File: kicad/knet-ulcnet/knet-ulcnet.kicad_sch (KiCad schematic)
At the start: 16 parts, among them U1 74LS157, U2 74LS00, U3 74LS139, U4 74LS86, U5 74LS74, U6 74LS74, U7 74LS123, U8 SN75176AP, U9 LM339

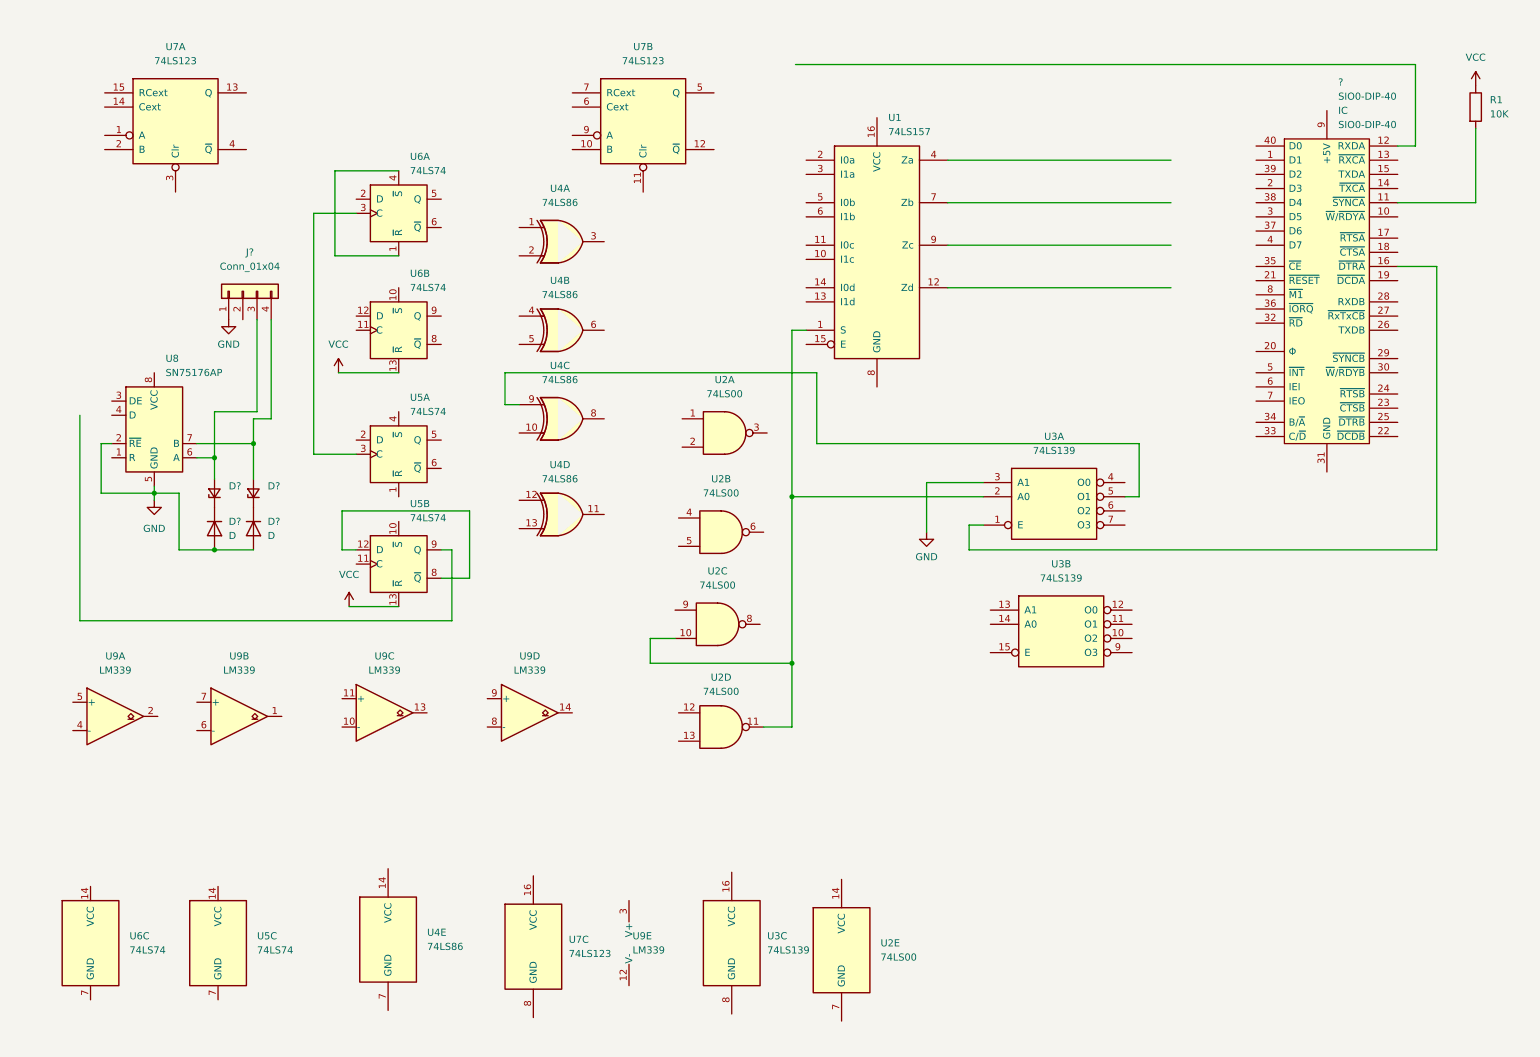
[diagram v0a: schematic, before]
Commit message: Update schematics etc for WEB-NT product
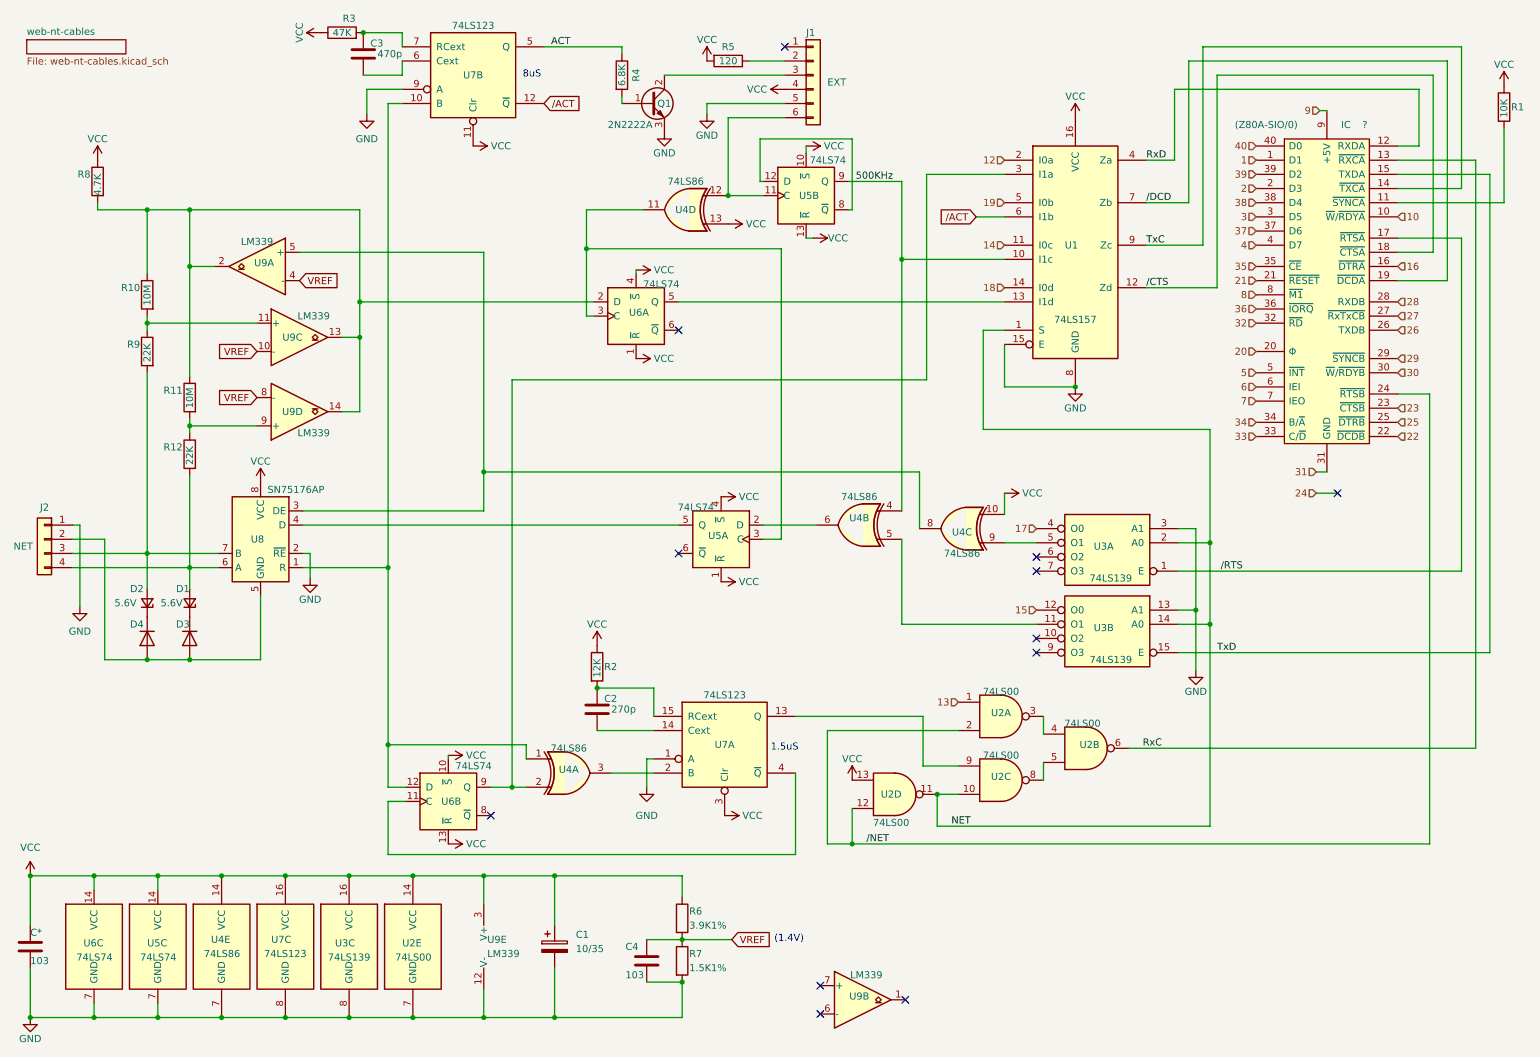
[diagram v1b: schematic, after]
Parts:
- added C*, C4: 103, symbol Device:C
- added C1: 10/35, symbol Device:C_Polarized
- added C2: 270p, symbol Device:C
- added C3: 470p, symbol Device:C
- added J1: EXT, symbol Connector_Generic:Conn_01x06
- added Q1: 2N2222A, symbol Device:Q_NPN_BCE
- added R10, R11: 10M, symbol Device:R
- added R12, R9: 22K, symbol Device:R
- added R2: 12K, symbol Device:R
- added R3: 47K, symbol Device:R
- added R4: 6.8K, symbol Device:R
- added R5: 120, symbol Device:R
- added R6: 3.9K1%, symbol Device:R
- added R7: 1.5K1%, symbol Device:R
- added R8: 4.7K, symbol Device:R
- ?: value SIO0-DIP-40 -> (none); Value_1 SIO0-DIP-40 -> (Z80A-SIO/0)
- D1, D2: renamed from D?; value (none) -> 5.6V
- D3, D4: renamed from D?; value D -> (none)
- J2: renamed from J?; value Conn_01x04 -> NET
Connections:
- net GND: now also U1.15 (E), U1.8 (GND), U2.7 (GND), U3.13 (A1), U3.8 (GND), U4.7 (GND), U5.7 (GND), U6.7 (GND), U7.1 (A), U7.8 (GND), U7.9 (A), U9.12 (V-), C*.2, C1.2, C4.2, J1.5 (Pin_5), Q1.3 (E), R7.2; no longer D3.2 (A), D4.2 (A), U8.5 (GND)
- net VCC: now also U1.16 (VCC), U2.13, U2.14 (VCC), U3.16 (VCC), U4.10, U4.13, U4.14 (VCC), U5.1 (~{R}), U5.10 (~{S}), U5.14 (VCC), U5.4 (~{S}), U6.1 (~{R}), U6.10 (~{S}), U6.14 (VCC), U6.4 (~{S}), U7.11 (Clr), U7.16 (VCC), U7.3 (Clr), U8.8 (VCC), U9.3 (V+), C*.1, C1.1, J1.4 (Pin_4), R2.1, R3.1, R5.2, R6.1, R8.1
- net NET: now reaches U1.1 (S), U2.10, U2.11, U3.2 (A0)
- net NET: now also U3.14 (A0)
- net 500KHz: now reaches U1.10 (I1c)
- net 500KHz: now also U4.4, U5.9 (Q)
- net 14: now reaches U1.11 (I0c)
- net /CTS: now reaches U1.12 (Zd)
- net /CTS: now also ?.18 (~{CTSA})
- net at U1.13 (I1d): now also U6.5 (Q)
- net 18: now reaches U1.14 (I0d)
- net 12: now reaches U1.2 (I0a)
- net at U1.3 (I1a): now also U4.2, U6.9 (Q)
- net RxD: now reaches U1.4 (Za)
- net RxD: now also ?.12 (RXDA)
- net 19: now reaches U1.5 (I0b)
- net /ACT: now reaches U1.6 (I1b)
- net /ACT: now also U7.12 (~{Q})
- net /DCD: now reaches U1.7 (Zb)
- net /DCD: now also ?.19 (~{DCDA})
- net TxC: now reaches U1.9 (Zc)
- net TxC: now also ?.14 (~{TXCA})
- net at D2.2 (A), U8.7 (B): now also J2.3 (Pin_3), R9.2; no longer J2.4 (Pin_4)
- net at U9.2: now also U6.2 (D), U9.13, U9.14, R10.1, R11.1, R8.2
- net VREF: now reaches U9.4 (-)
- net VREF: now also U9.10 (-), U9.8 (-), C4.1, R6.2, R7.1
- net at U9.5 (+): now also U4.8, U8.3 (DE)
- net at U3.11 (O1): now also U4.5
- net 15: now reaches U3.12 (O0)
- net TxD: now reaches U3.15 (E)
- net TxD: now also ?.15 (TXDA)
- net /NET: now reaches U2.12
- net /NET: now also ?.24 (~{RTSB}), U2.2
- net at U7.13 (Q): now also U2.9
- net at U7.14 (Cext): now also C2.2
- net at U7.15 (RCext): now also C2.1, R2.2
- net at U7.2 (B): now also U4.3
- net at U7.4 (~{Q}): now also U6.11 (C)
- net 13: now reaches U2.1
- net at U2.3: now also U2.4
- net at U4.11: now also U5.3 (C), U6.3 (C)
- net at U4.12: now also U5.11 (C), J1.6 (Pin_6)
- net at U6.12 (D): now also U4.1, U7.10 (B), U8.1 (R)
- net ACT: now reaches U7.5 (Q)
- net ACT: now also R4.1
- net at U7.6 (Cext): now also C3.2
- net at U7.7 (RCext): now also C3.1, R3.2
- net 1: now reaches ?.1 (D1)
- net 10: now reaches ?.10 (~{W}/~{RDYA})
- net RxC: now reaches ?.13 (~{RXCA})
- net RxC: now also U2.6
- net 16: now reaches ?.16 (~{DTRA})
- net 16: no longer U3.1 (E)
- net /RTS: now reaches ?.17 (~{RTSA})
- net /RTS: now also U3.1 (E)
- net 2: now reaches ?.2 (D3)
- net 20: now reaches ?.20 (Φ)
- net 21: now reaches ?.21 (~{RESET})
- net 22: now reaches ?.22 (~{DCDB})
- net 23: now reaches ?.23 (~{CTSB})
- net 25: now reaches ?.25 (~{DTRB})
- net 26: now reaches ?.26 (TXDB)
- net 27: now reaches ?.27 (~{RxTxCB})
- net 28: now reaches ?.28 (RXDB)
- net 29: now reaches ?.29 (~{SYNCB})
- net 3: now reaches ?.3 (D5)
- net 30: now reaches ?.30 (~{W}/~{RDYB})
- net 31: now reaches ?.31 (GND)
- net 32: now reaches ?.32 (~{RD})
- net 33: now reaches ?.33 (C/~{D})
- net 34: now reaches ?.34 (B/~{A})
- net 35: now reaches ?.35 (~{CE})
- net 36: now reaches ?.36 (~{IORQ})
- net 37: now reaches ?.37 (D6)
- net 38: now reaches ?.38 (D4)
- net 39: now reaches ?.39 (D2)
- net 4: now reaches ?.4 (D7)
- net 40: now reaches ?.40 (D0)
- net 5: now reaches ?.5 (~{INT})
- net 6: now reaches ?.6 (IEI)
- net 7: now reaches ?.7 (IEO)
- net 8: now reaches ?.8 (~{M1})
- net 9: now reaches ?.9 (+5V)
- net at U4.6: now also U5.2 (D)
- net at J2.2 (Pin_2): now also D3.2 (A), D4.2 (A), U8.5 (GND)
- net at D1.2 (A), U8.6 (A): now also J2.4 (Pin_4), R12.2; no longer J2.3 (Pin_3)
- net at U2.5: now also U2.8
- net at U9.11 (+): now also R10.2, R9.1
- net at U8.4 (D): now also U5.5 (Q)
- net at U9.9 (+): now also R11.2, R12.1
- net 17: now reaches U3.4 (O0)
- new net: Q1.1 (B), R4.2
- new net: J1.3 (Pin_3), Q1.2 (C)
- new net: J1.2 (Pin_2), R5.1
- no-connect marks 0 -> 12
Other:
- added sheet web-nt-cables (web-nt-cables.kicad_sch)
- note added: "(1.4V)"
- note added: "1.5uS"
- note added: "8uS"
- moved on the sheet: D1, D2, D3, D4, J2, R1, U1, U2A, U2B, U2C, U2D, U2E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
